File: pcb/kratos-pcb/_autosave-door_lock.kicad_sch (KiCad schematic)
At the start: 8 parts, among them IC1 SN74HC595N, Q2 2N2222A, Q3 2N2222A, U2 74HC595

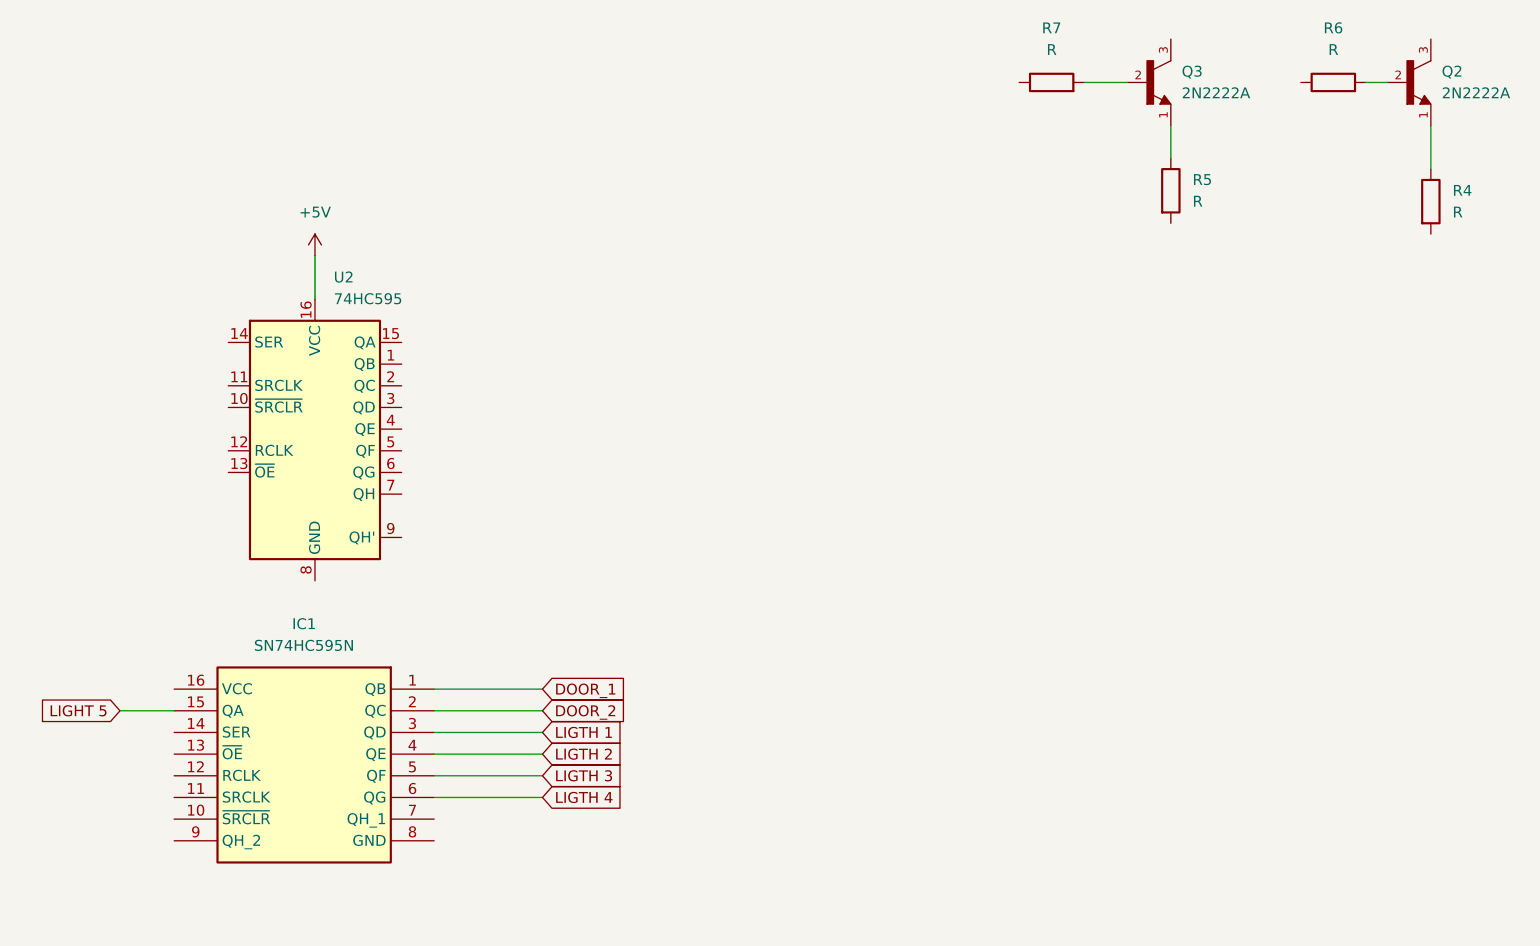
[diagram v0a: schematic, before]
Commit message: ### Added
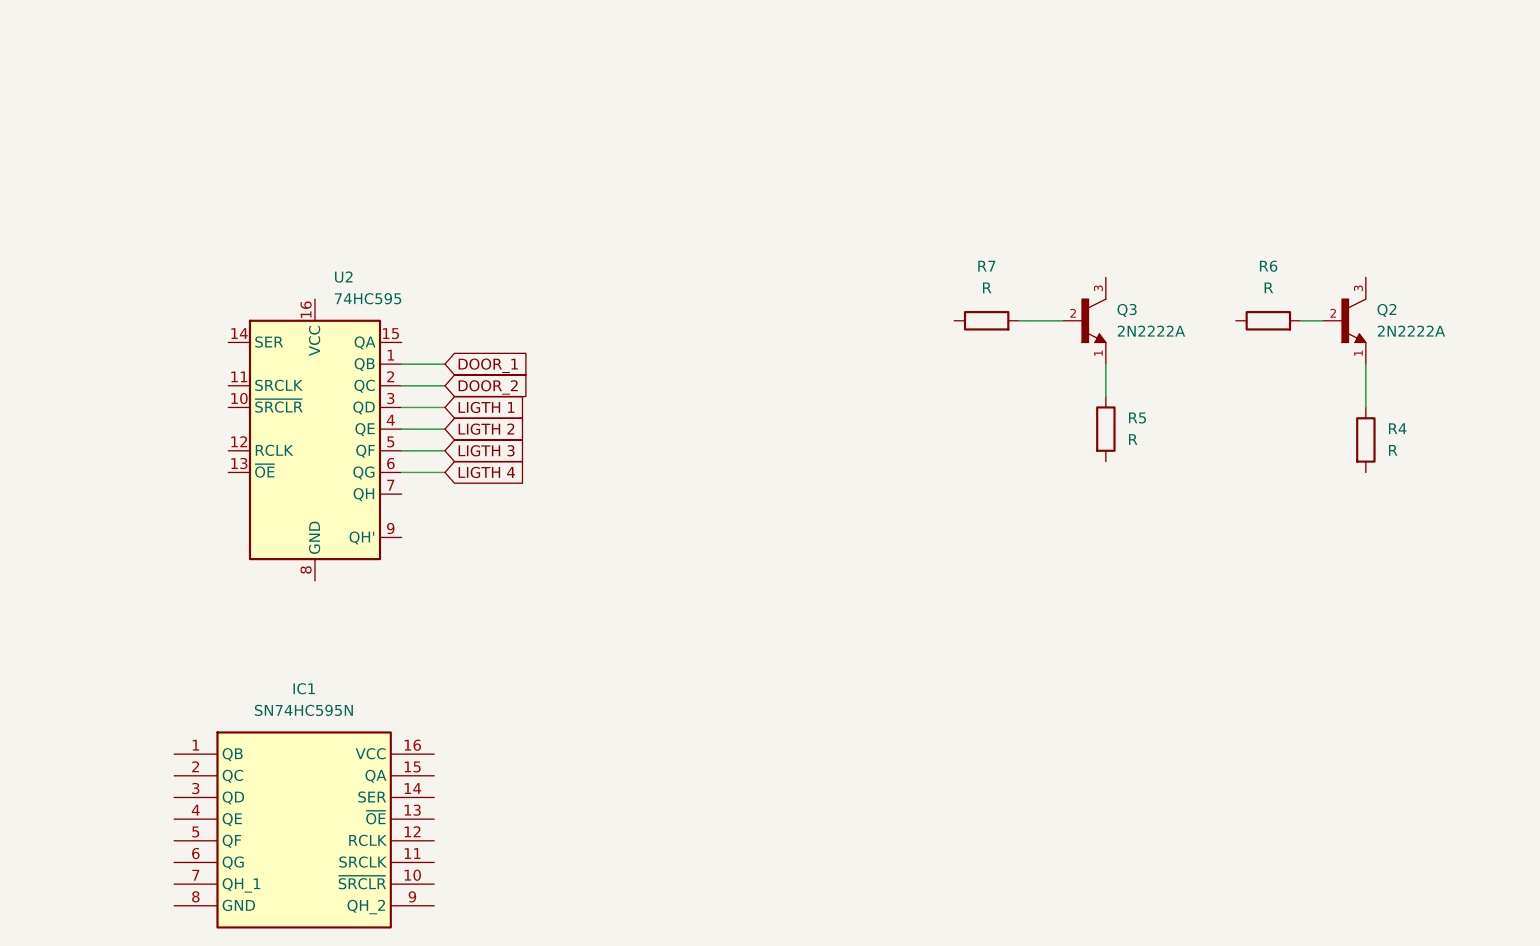
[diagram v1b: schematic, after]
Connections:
- net DOOR_1: now also U2.1 (QB); no longer IC1.1 (QB)
- net DOOR_2: now also U2.2 (QC); no longer IC1.2 (QC)
- net LIGTH 1: now also U2.3 (QD); no longer IC1.3 (QD)
- net LIGTH 2: now also U2.4 (QE); no longer IC1.4 (QE)
- net LIGTH 3: now also U2.5 (QF); no longer IC1.5 (QF)
- net LIGTH 4: now also U2.6 (QG); no longer IC1.6 (QG)
- net +5V: no longer names the net of U2.16 (VCC)
- net LIGHT 5: no longer names the net of IC1.15 (QA)
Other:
- moved on the sheet: IC1, Q2, Q3, R4, R5, R6, R7
